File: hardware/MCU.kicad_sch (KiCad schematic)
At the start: 48 parts, among them IC1 TCAN330DCNT, J1 BM04B-GHS-TBT_LF__SN__N_, J2 USB_C_Receptacle_USB2.0_16P, J3 Conn_01x02_Socket, J4 Conn_01x04_Pin, J5 BM04B-GHS-TBT_LF__SN__N_, SW1 SW_SPDT, SW2 SW_SPDT, U2 ME6211C33M5, U3 STM32G431CBU6, Y1 ECS-80-20-5PX-TR

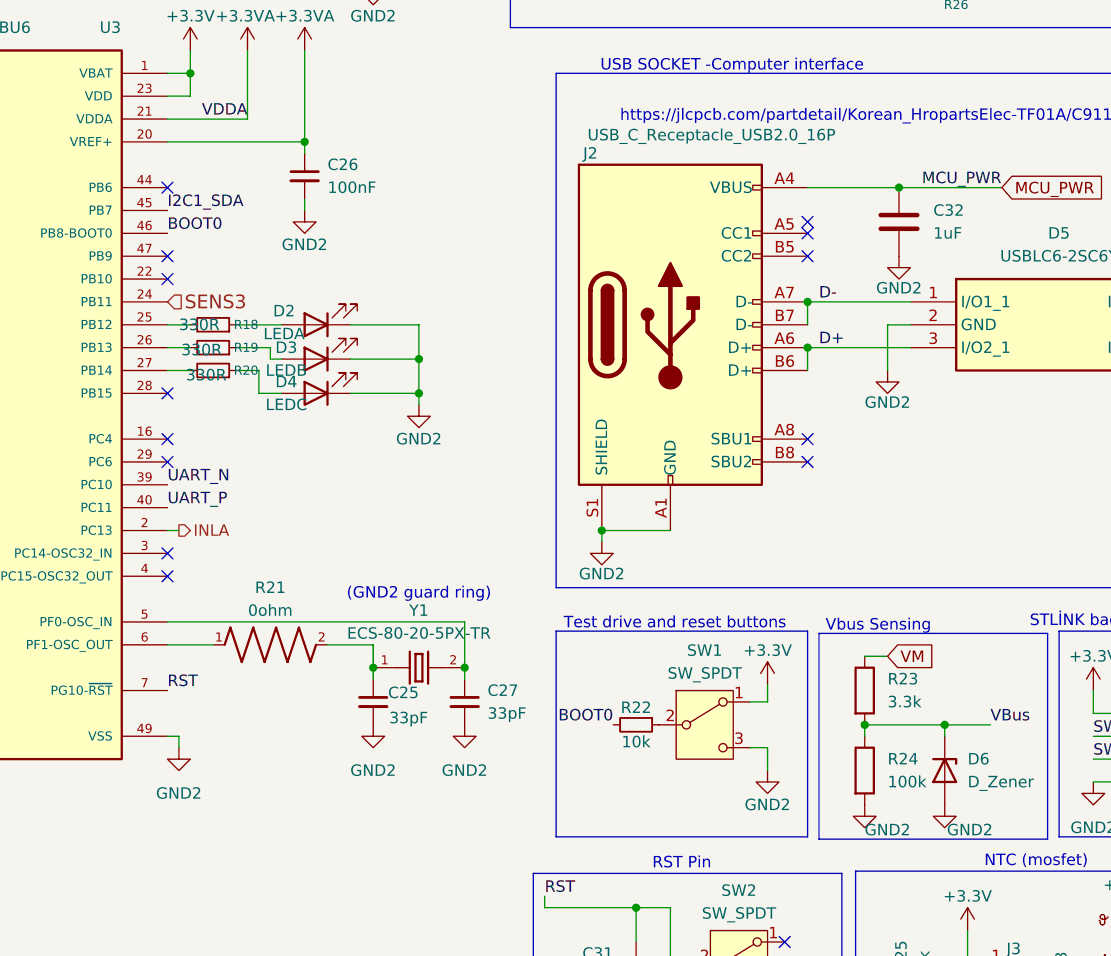
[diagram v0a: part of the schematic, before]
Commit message: final project board layout is in this commit
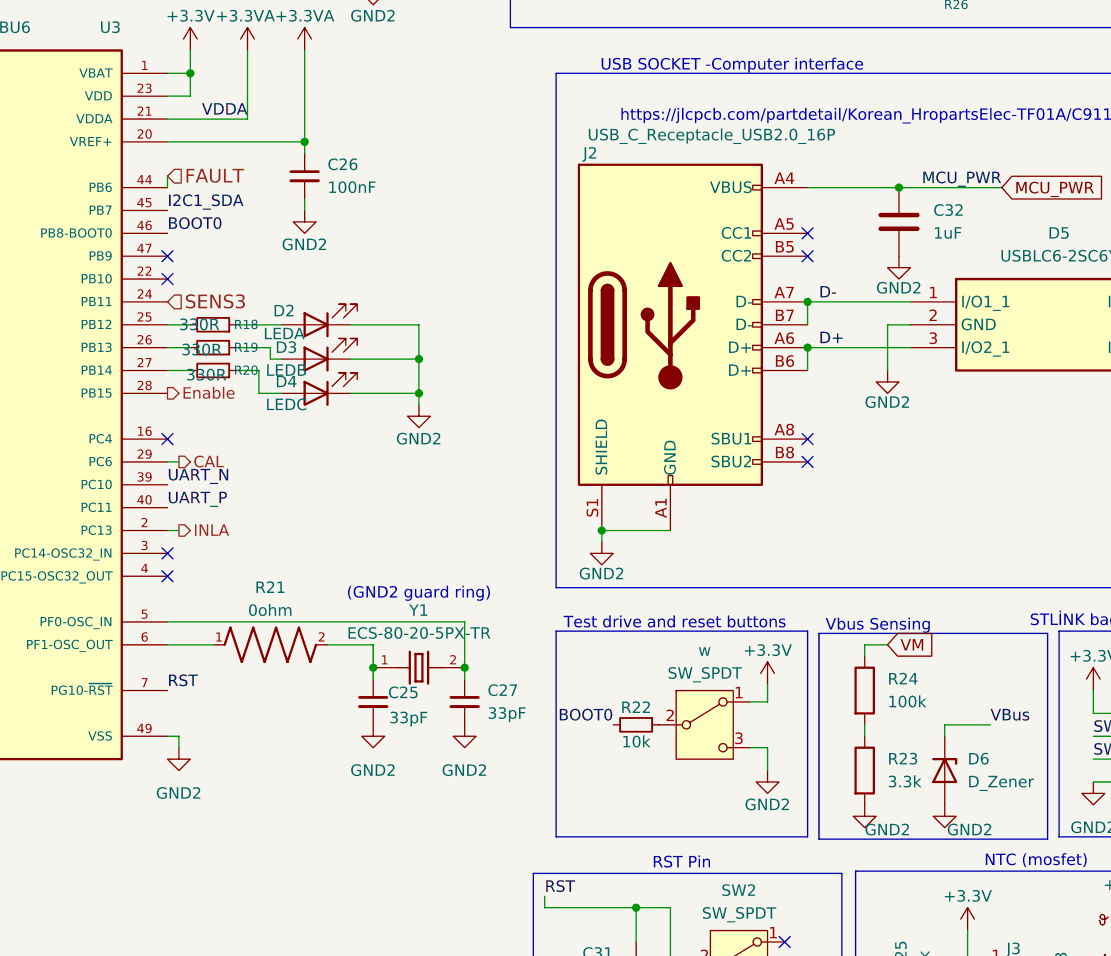
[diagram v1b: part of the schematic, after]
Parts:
- renumbered SW1 to w
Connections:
- net GND2: now also R23.2; no longer R24.2
- net VBus: no longer R23.2, R24.1
- net VM: now also R24.1; no longer R23.1
- net Enable: now reaches U3.28 (PB15)
- net CAL: now reaches U3.29 (PC6)
- net FAULT: now reaches U3.44 (PB6)
- new net: R23.1, R24.2
- no-connect marks 21 -> 17
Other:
- moved on the sheet: R23, R24
